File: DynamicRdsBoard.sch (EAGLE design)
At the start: 28 parts, among them Q1 FDP120N10, Q2 FDP120N10, U1 ADUM3223ARZ, X1 1751248, X2 1751280

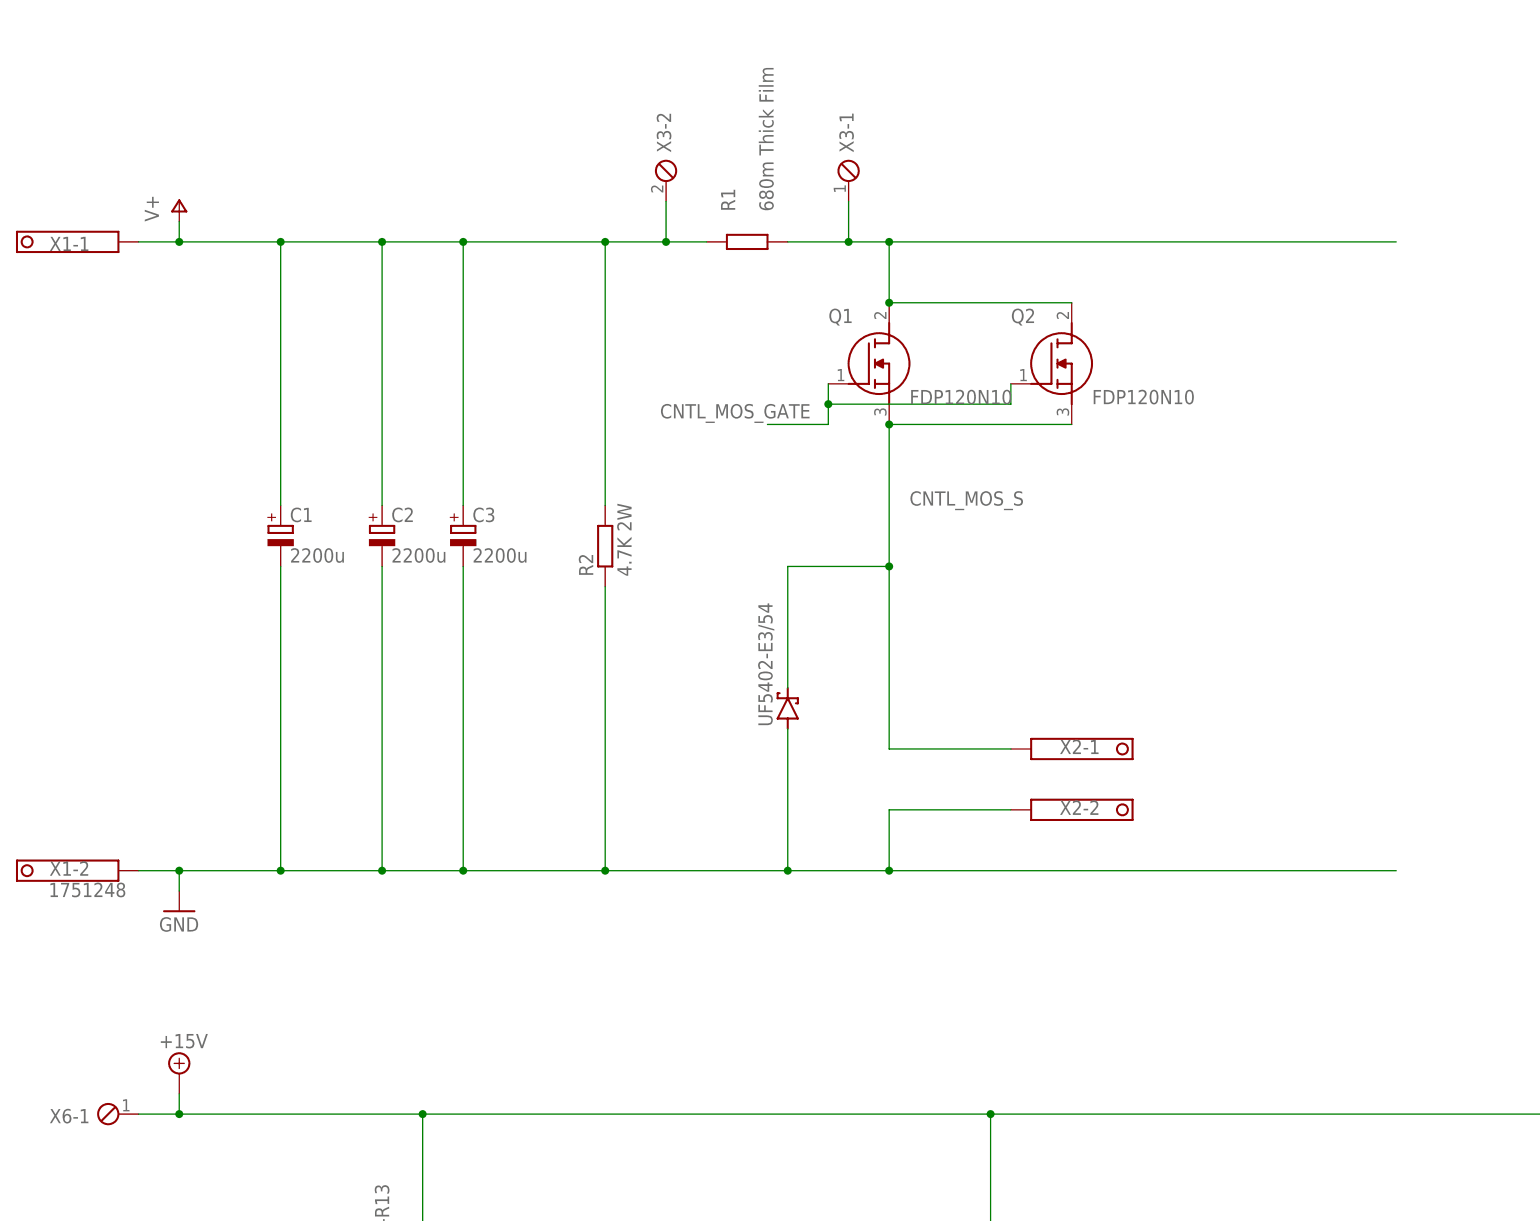
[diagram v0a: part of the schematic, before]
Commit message: Friday work commit
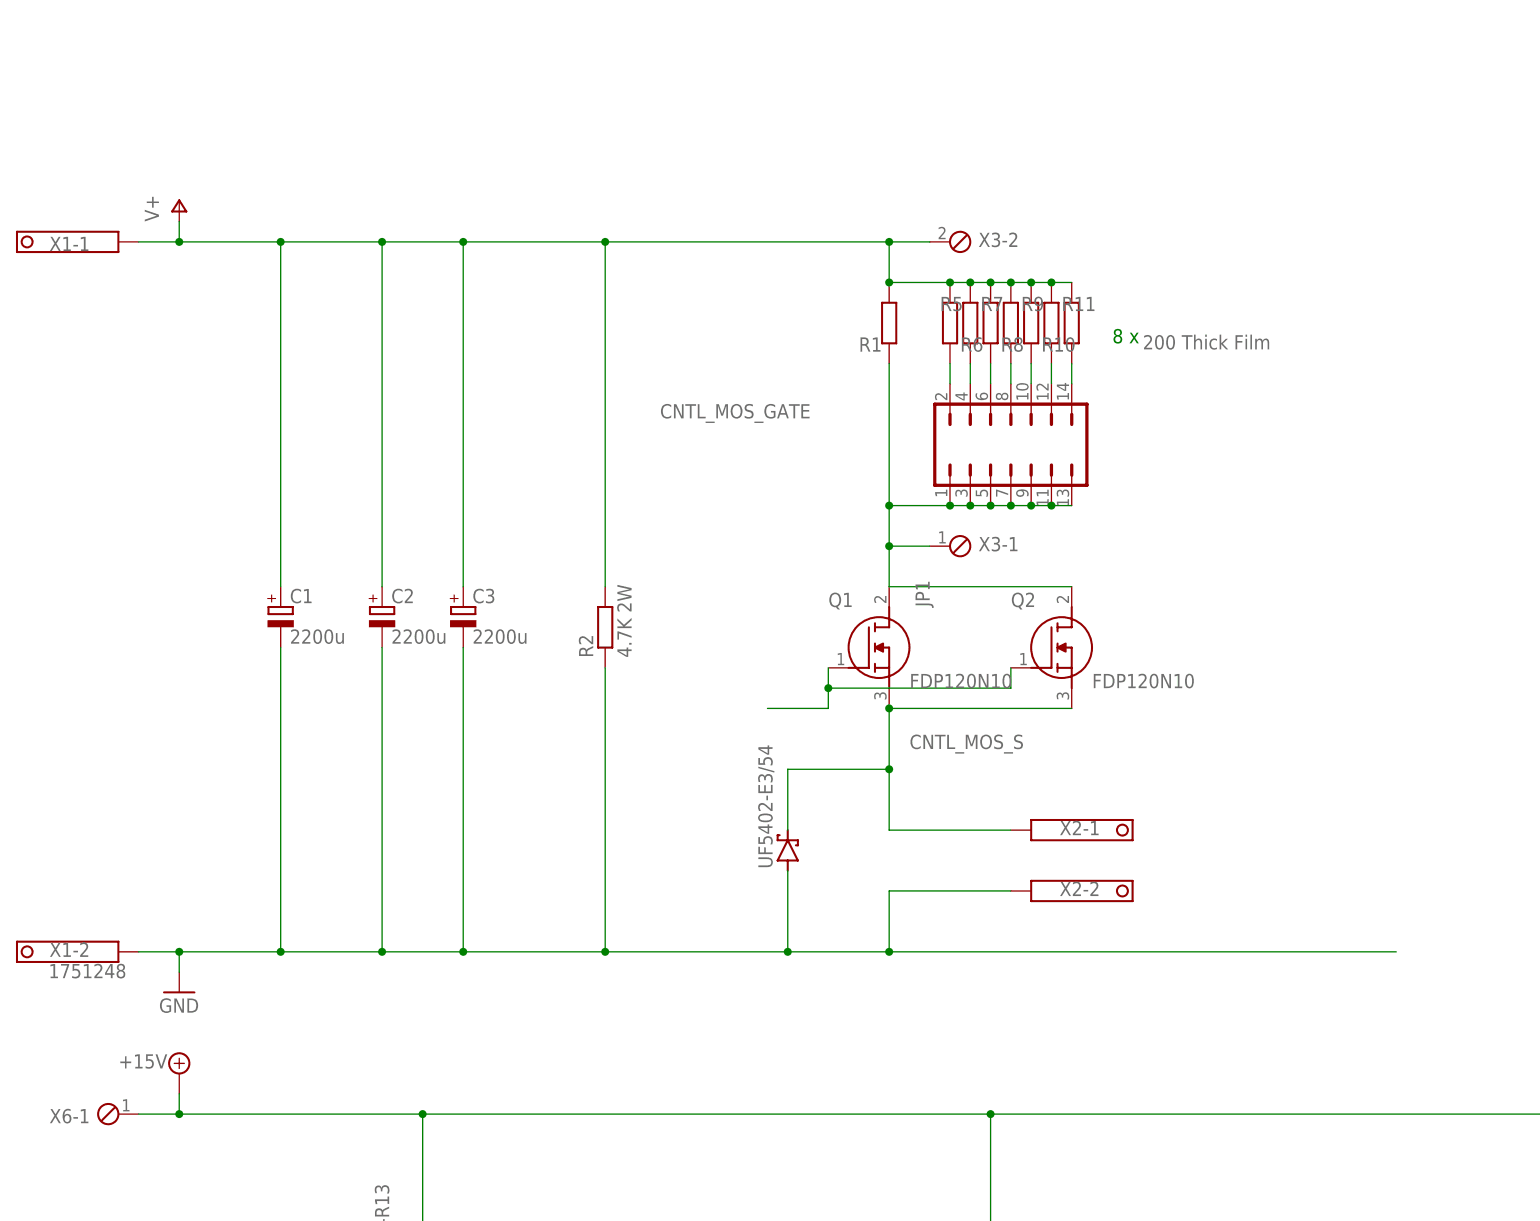
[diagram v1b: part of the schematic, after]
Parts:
- added JP1: (no value), jumper:JP7Q
- added R10, R11, R5, R6, R7, R8, R9: 200 Thick Film, rcl:R-EU_R1206
- R1: value 680m Thick Film -> 200 Thick Film; device rcl:R-EU_R1210 -> rcl:R-EU_R1206
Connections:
- new net N$2: JP1.2, R5.1
- new net N$3: JP1.4, R6.1
- new net N$4: JP1.6, R7.1
- new net N$5: JP1.8, R8.1
- new net N$6: JP1.10, R9.1
- new net N$7: JP1.12, R10.1
- new net N$8: JP1.14, R11.1
- net N$1: now also JP1.1, JP1.11, JP1.13, JP1.3, JP1.5, JP1.7, JP1.9
- net V+: now also R10.2, R11.2, R5.2, R6.2, R7.2, R8.2, R9.2
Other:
- note added: "8 x"
- moved on the sheet: C1, C2, C3, Q1, Q2, R1, R2, UF5402-E3/54, X1-2, X2-1, X2-2, X3-1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
